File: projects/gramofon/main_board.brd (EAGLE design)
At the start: 290 x 99 mm, 23 parts

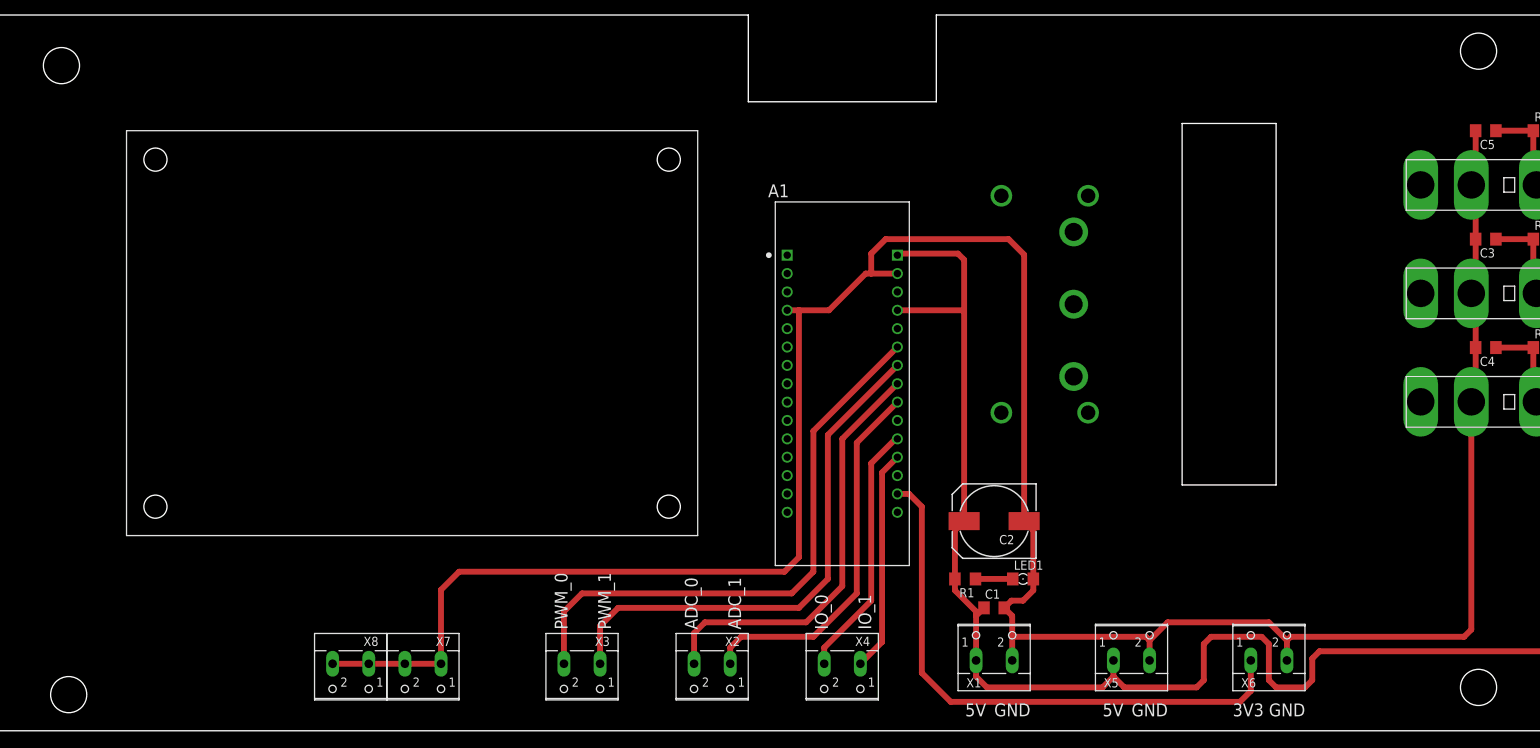
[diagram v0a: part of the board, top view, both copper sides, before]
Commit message: gramofon update
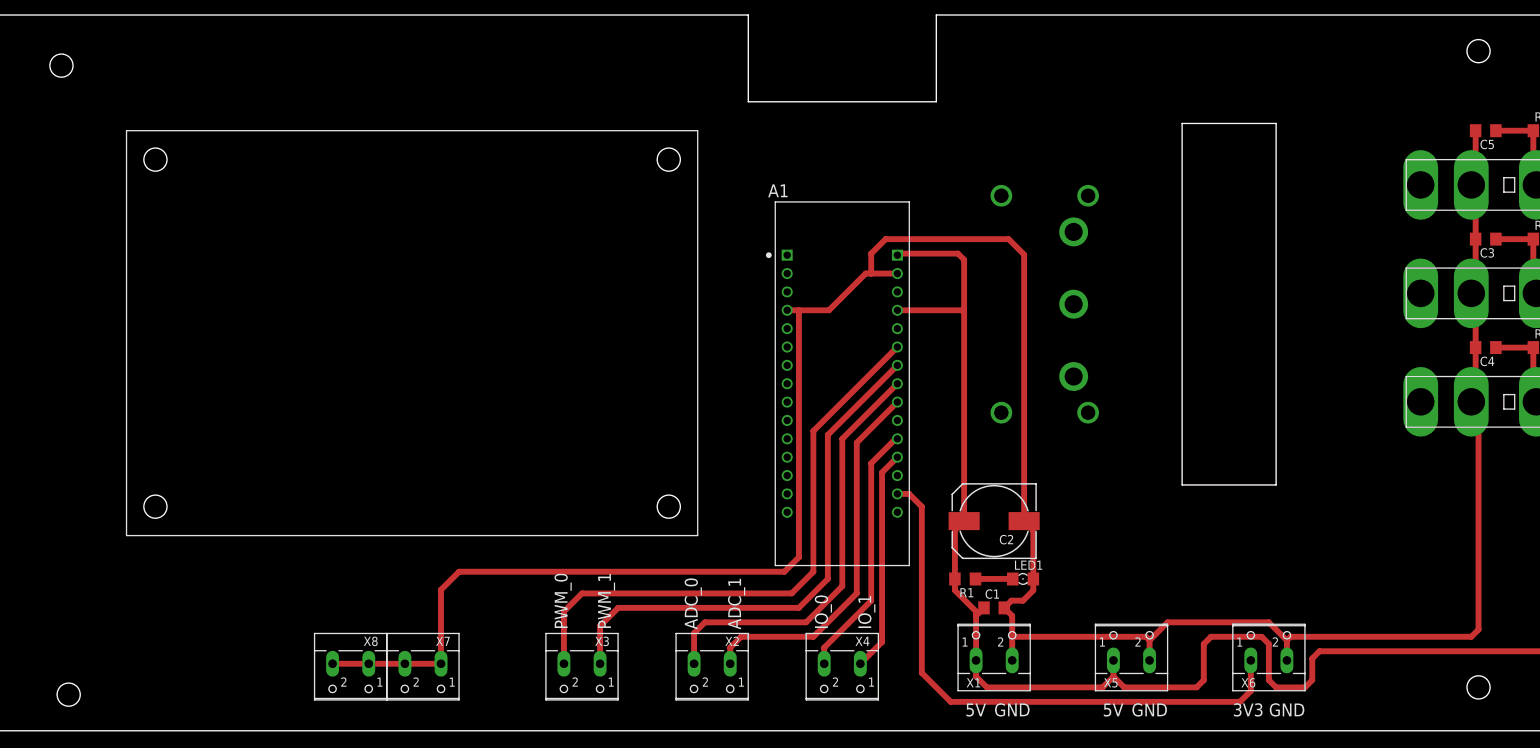
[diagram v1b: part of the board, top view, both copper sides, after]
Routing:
- net GND: track 355.6 -> 357.0 mm
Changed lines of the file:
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@@
 <wire x1="222" y1="34" x2="222" y2="84" width="0.1524" layer="20"/>
 <wire x1="222" y1="84" x2="235" y2="84" width="0.1524" layer="20"/>
-<hole x="263" y="94" drill="5"/>
-<hole x="263" y="6" drill="5"/>
-<hole x="68" y="5" drill="5"/>
 <dimension x1="263" y1="94" x2="290" y2="94" x3="276.5" y3="89" textsize="1.778" layer="47"/>
 <dimension x1="263" y1="94" x2="263" y2="99" x3="258" y3="96.5" textsize="1.778" layer="47"/>
@@
 <dimension x1="222" y1="34" x2="222" y2="84" x3="240" y3="59" textsize="1.778" layer="47"/>
 <dimension x1="222" y1="84" x2="235" y2="84" x3="228.5" y3="87" textsize="1.778" layer="47"/>
-<hole x="67" y="92" drill="5"/>
 <dimension x1="67" y1="92" x2="57" y2="92" x3="62" y3="86" textsize="1.778" layer="47"/>
 <dimension x1="67" y1="92" x2="67" y2="99" x3="74" y3="95.5" textsize="1.778" layer="47"/>
@@
 <text x="143" y="14" size="1.778" layer="25" rot="R90">PWM_1</text>
 <wire x1="57" y1="86" x2="57" y2="0" width="0.8128" layer="25"/>
+<hole x="263" y="94" drill="3.2"/>
+<hole x="263" y="6" drill="3.2"/>
+<hole x="68" y="5" drill="3.2"/>
+<hole x="67" y="92" drill="3.2"/>
 </plain>
 <attributes>
@@
 <wire x1="262.6" y1="46.1" x2="262" y2="45.5" width="0.8128" layer="1"/>
 <wire x1="236.5" y1="12.5" x2="237" y2="13" width="0.8128" layer="1"/>
-<wire x1="237" y1="13" x2="261" y2="13" width="0.8128" layer="1"/>
-<wire x1="261" y1="13" x2="262" y2="14" width="0.8128" layer="1"/>
-<wire x1="262" y1="14" x2="262" y2="45.5" width="0.8128" layer="1"/>
+<wire x1="237" y1="13" x2="262" y2="13" width="0.8128" layer="1"/>
+<wire x1="262" y1="13" x2="263" y2="14" width="0.8128" layer="1"/>
+<wire x1="263" y1="44.5" x2="263" y2="14" width="0.8128" layer="1"/>
+<wire x1="263" y1="44.5" x2="262" y2="45.5" width="0.8128" layer="1"/>
 <wire x1="167.38" y1="58.16" x2="169" y2="58.16" width="0.8128" layer="1"/>
 <wire x1="169" y1="58.16" x2="173.16" y2="58.16" width="0.8128" layer="1"/>
